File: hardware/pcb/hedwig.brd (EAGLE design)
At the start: 76.2 x 68.5 mm, 75 parts, among them IC1 MPL3115A2LGA, J1 DX07B024JJ1R1500, P1 JTAG-10MINI, Q1 16MHz, Q2 IRLML6402, U1 NRF24L01SMD, U2 TEXAS_INSTRUMENTS_TLC59731DRT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, U3 FT232RQ, U5 ADP2302, U7 9DoF IMU, X1 8M, X2 32.768

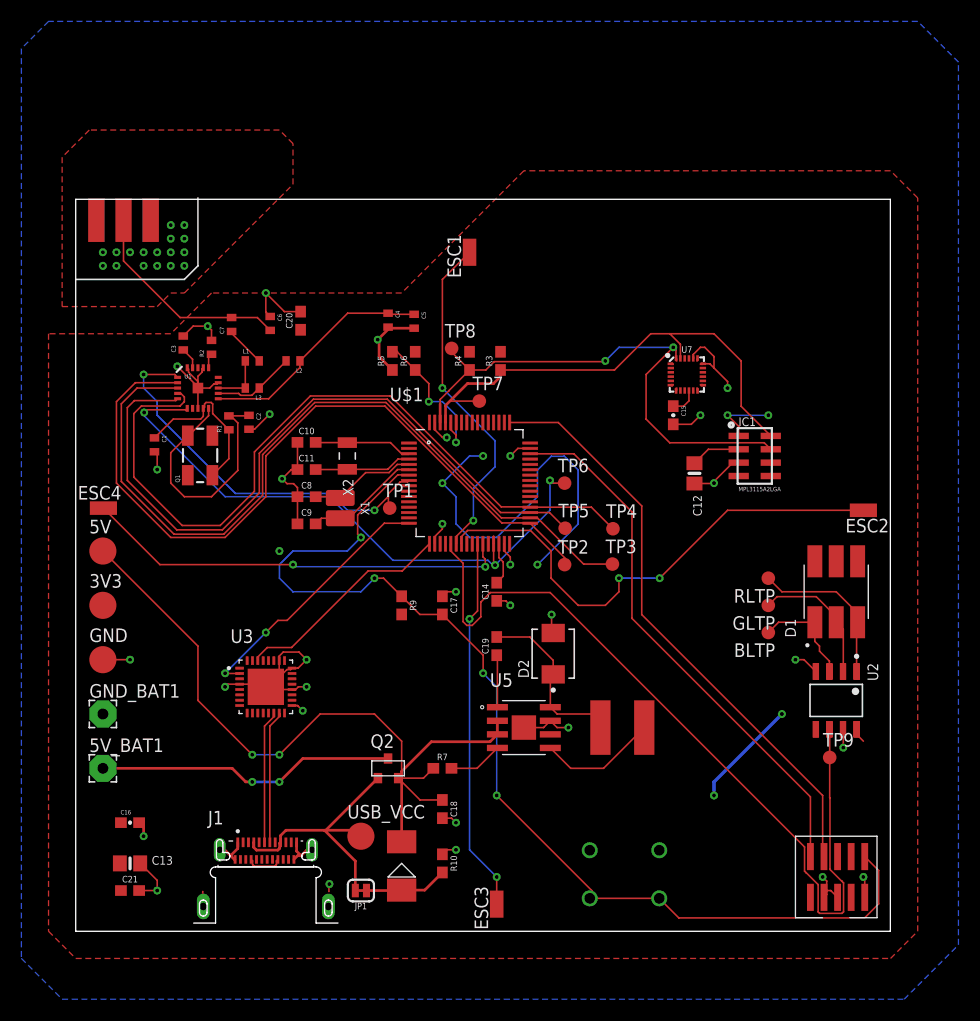
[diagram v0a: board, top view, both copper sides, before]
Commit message: updated schematic and pcb
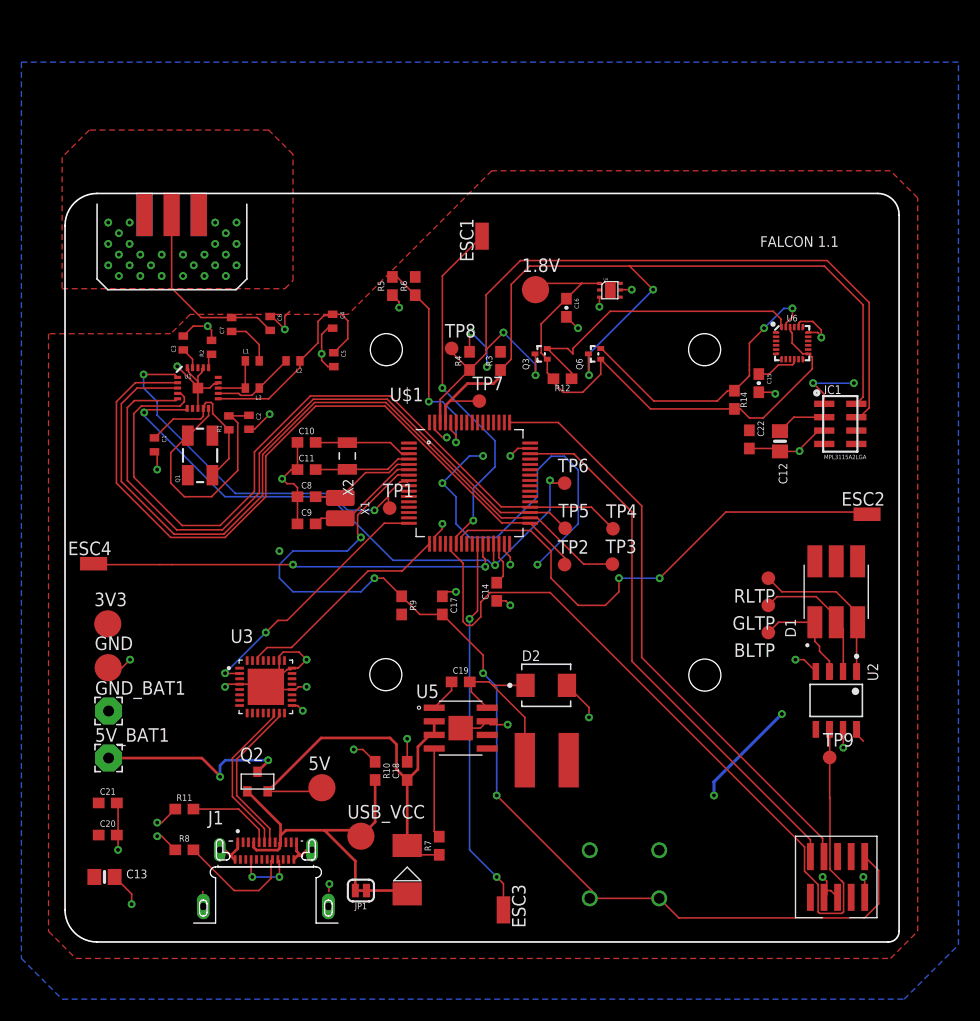
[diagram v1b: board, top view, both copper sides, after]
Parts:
- removed U$6: DIODE, falcon:SMB
- removed U7: 9DoF IMU, SparkFun-Sensors:QFN24-3X3
- added 1.8V: TPB2,54, testpad:B2,54
- added C22: 47uF, SparkFun-Capacitors:0603@1
- added D3: SURS8360BT3G, falcon:SMB
- added Q3, Q6: 20V/0.2A/8MHz/1.2Ω/1Vth, SparkFun-DiscreteSemi:SOT-416FL
- added R11, R8: 5.1k, SparkFun-Resistors:0603
- added R12, R14: 2.49k, SparkFun-Resistors:0603
- added U4: TPS7A26-1.8, falcon:WSON
- added U6: 9DoF IMU, SparkFun-Sensors:QFN24-3X3
- C10, C11: value 1.5pF -> 0.1uF
- C14: value 2.2uF -> 0.1uF
- C17: value 100nF -> 0.1uF
- C18, C19, C20, C21: device SparkFun-Capacitors:0603 -> SparkFun-Capacitors:0603@1
- C8, C9: value 8.2pF -> 0.1uF
- moved C16 63.1 mm to (45.9, 58.3), turned to 270 degrees
- moved C20 51.4 mm to (3.00, 9.00), turned to 0 degrees
- moved 5V 30.2 mm to (23.0, 13.4)
- moved Q2 12.3 mm to (17.0, 14.0)
- moved R10 10.7 mm to (28.0, 15.0)
- moved C12 8.54 mm to (65.9, 45.8)
- moved C15 8.54 mm to (63.9, 51.3)
- moved IC1 8.54 mm to (71.5, 47.5)
- moved C21 8.45 mm to (3.00, 12.0)
- moved C5 8.32 mm to (24.1, 53.5)
- moved U$4 7.70 mm to (45.0, 16.0)
- moved R7 7.25 mm to (34.0, 8.00), turned to 90 degrees
- moved R5 7.00 mm to (29.6, 60.3)
- moved R6 7.00 mm to (31.8, 60.3)
- moved U5 5.91 mm to (36.0, 19.0)
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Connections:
- new net 1P8V: 1.8V.TP, C16.1, Q3.1, Q6.1, R12.2, R14.2, U4.1, U6.13, U6.22
- new net N$15: J1.B5, R8.2
- new net N$26: J1.A5, R11.2
- new net SENSOR_SCL_LV: Q6.2, R14.1, U6.23
- new net SENSOR_SDA_LV: Q3.2, R12.1, U6.24
- net +3V3: now also C22.1, U4.4, U4.6; no longer C16.1, U7.13, U7.22
- net +5V: now also D3.@2; no longer U$6.@2
- net ADSD_STUB: now also U6.9; no longer U7.9
- net GND: now also C22.2, R11.1, R8.1, U4.3, U4.5, U6.18, U6.20; no longer U7.18, U7.20
- net REGOUT: now also U6.10; no longer U7.10
- net SENSOR_SCL: now also Q6.3; no longer U7.23
- net SENSOR_SDA: now also Q3.3; no longer U7.24
- net USB_VCC: now also D3.@1; no longer U$6.@1
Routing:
- net 1P8V: track 0.00 -> 53.5 mm
- net SENSOR_SCL: track 47.6 -> 80.5 mm, vias 0 -> 2
- net +5V: track 72.1 -> 39.6 mm, vias 2 -> 0
- net SENSOR_SDA_LV: track 0.00 -> 29.0 mm
- net SENSOR_SCL_LV: track 0.00 -> 27.4 mm, vias 0 -> 2
- net SENSOR_SDA: track 50.4 -> 76.6 mm
- net N$15: track 0.00 -> 11.1 mm
- net N$25: track 28.1 -> 18.4 mm
- net N$26: track 0.00 -> 8.13 mm
- net GND: track 129.4 -> 137.1 mm, vias 50 -> 67
- net N$16: track 14.0 -> 21.0 mm
- net +3V3: track 65.7 -> 60.2 mm, vias 7 -> 9
- net N$23: track 5.08 -> 8.44 mm
- net N$22: track 12.5 -> 15.1 mm
- net N$21: track 12.5 -> 15.0 mm
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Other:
- board size 76.2 x 68.5 mm -> 78 x 70 mm
- board text added: "FALCON 1.1"
